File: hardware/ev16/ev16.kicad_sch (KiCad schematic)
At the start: 175 parts, among them CN1 Conn_05x02_Female, CN2 PJ-242, J1 USB_C_Receptacle, J10 Conn_01x03_Pin, J11 Conn_02x05_Counter_Clockwise, J2 Conn_01x02_Socket, J3 AudioJack4, J4 Conn_02x03_Odd_Even, J5 Conn_02x03_Odd_Even, J6 Conn_02x05_Counter_Clockwise, J7 Conn_02x05_Counter_Clockwise, J8 Conn_02x05_Counter_Clockwise, J9 Conn_02x05_Counter_Clockwise, Q1 2N7002, Q2 2N7002, Q3 2N7002, SW1 SW_SPDT, SW2 SW_Push, SW3 SW_Push, SW4 SW_Push, SW5 SW_Push, SW6 SW_Push, SW7 SW_Push, SW8 SW_Push, U1 BQ21040DBV, U10 STM32F405RGTx, U2 USBLC6-2P6, U3 STM32F072CBTx, U4 CH340C, U5 TPS63060, U6 WM8960CGEFL/RV, U7 ESP32-S3-WROOM-1, U8 M24C02-RMN6TP, Y1 Crystal_GND24

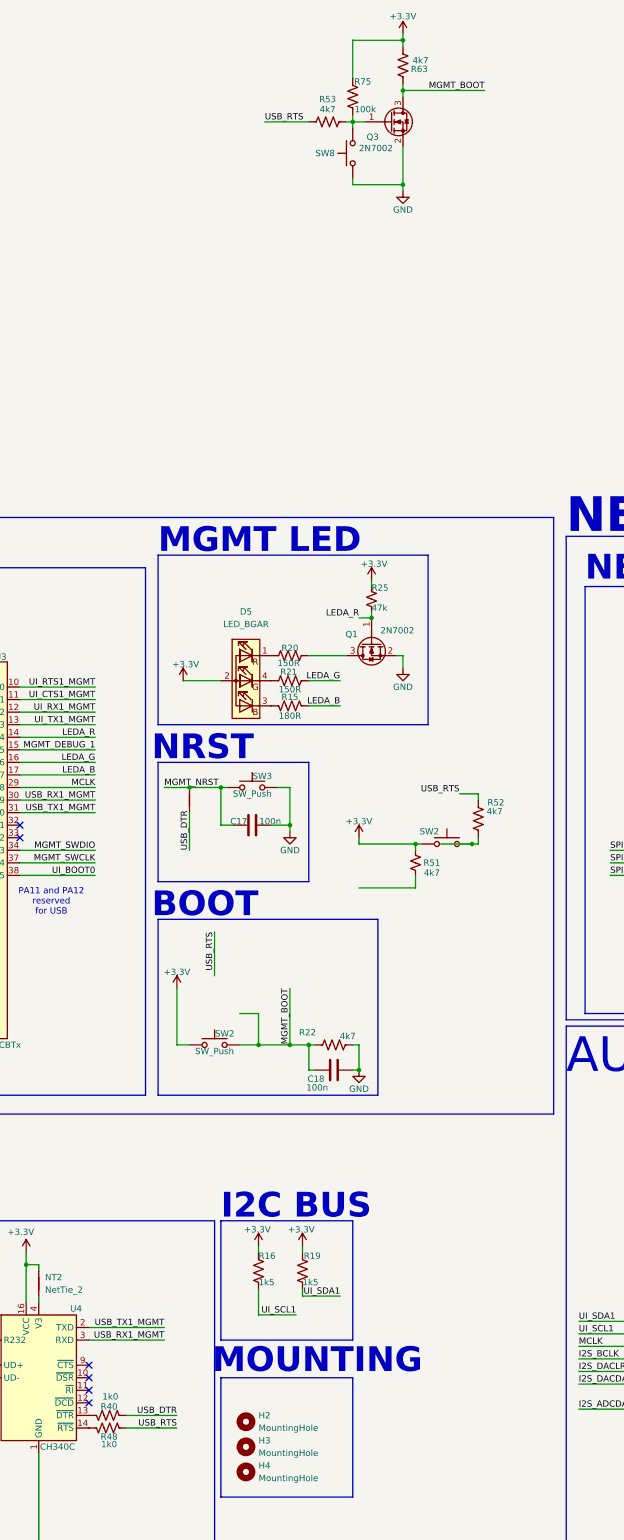
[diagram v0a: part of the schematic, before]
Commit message: production generator push
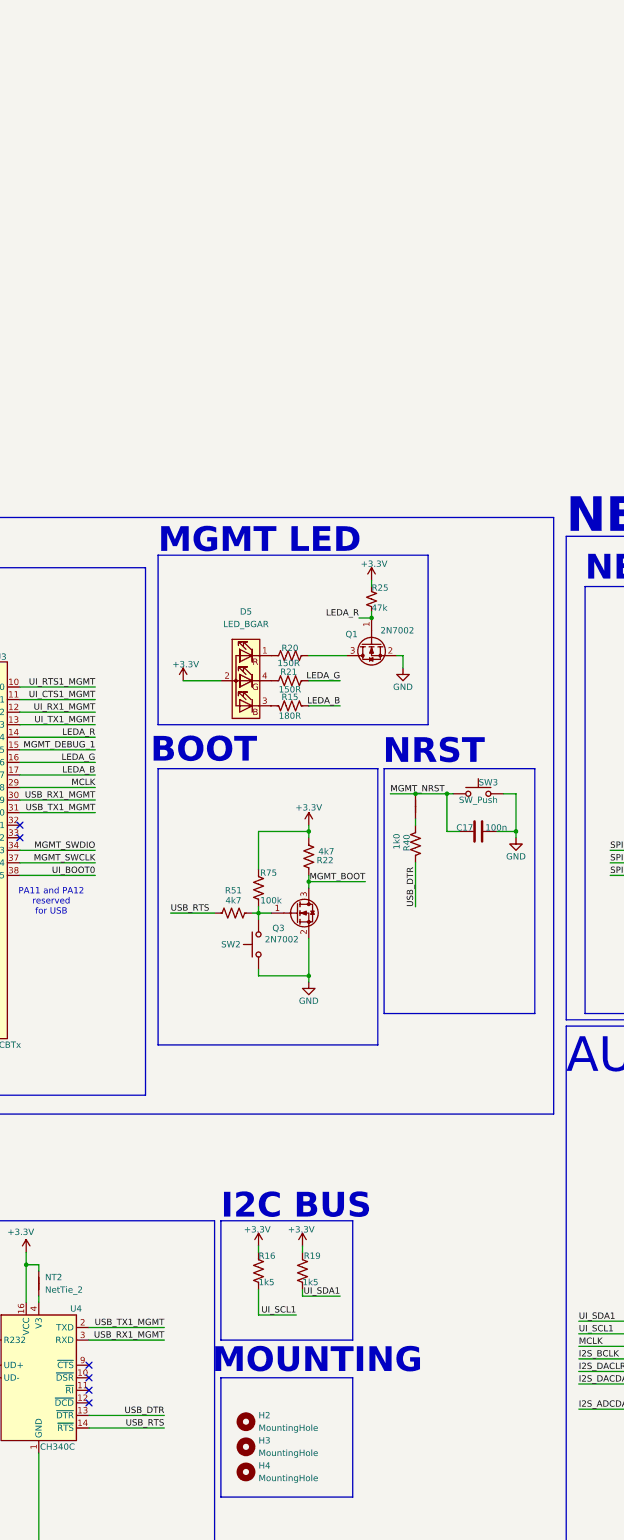
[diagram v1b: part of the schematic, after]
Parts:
- removed C18: 100n, Capacitor_SMD:C_0402_1005Metric, symbol Device:C
- removed R22, R52, R53: 4k7, Resistor_SMD:R_0402_1005Metric, symbol Device:R_US
- removed R48: 1k0, Resistor_SMD:R_0402_1005Metric, symbol Device:R_US
- removed R51: 4k7, Resistor_SMD:R_0402_1005Metric, symbol Device:R_Small_US
- removed SW2 (x2): SW_Push, Hactar_Footprints:KEY-SMD_4P-L4.2-W3.2-P2.20-LS4.6, symbol Hactar_Symbols:SW_Push_4C
- added R51: 4k7, Resistor_SMD:R_0402_1005Metric, symbol Device:R_US
- renumbered R63 to R22, SW8 to SW2
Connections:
- net USB_DTR: now also R40.2, U4.13 (~{DTR}); no longer NT3.1, R40.1
- net USB_RTS: now also U4.14 (~{RTS}), R51.1
- net at Q3.1 (G), R75.1, SW2.3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: now also R51.2
- new net: NT3.1, R40.1
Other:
- moved on the sheet: C17, Q3, R22, R40, R75, SW2, SW3
